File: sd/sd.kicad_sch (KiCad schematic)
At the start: 18 parts, among them J1 Micro_SD_Card_Det2, J3 STM32WORLD_BOARD, J4 STM32WORLD_CONNECTOR_1, J5 STM32WORLD_CONNECTOR_2

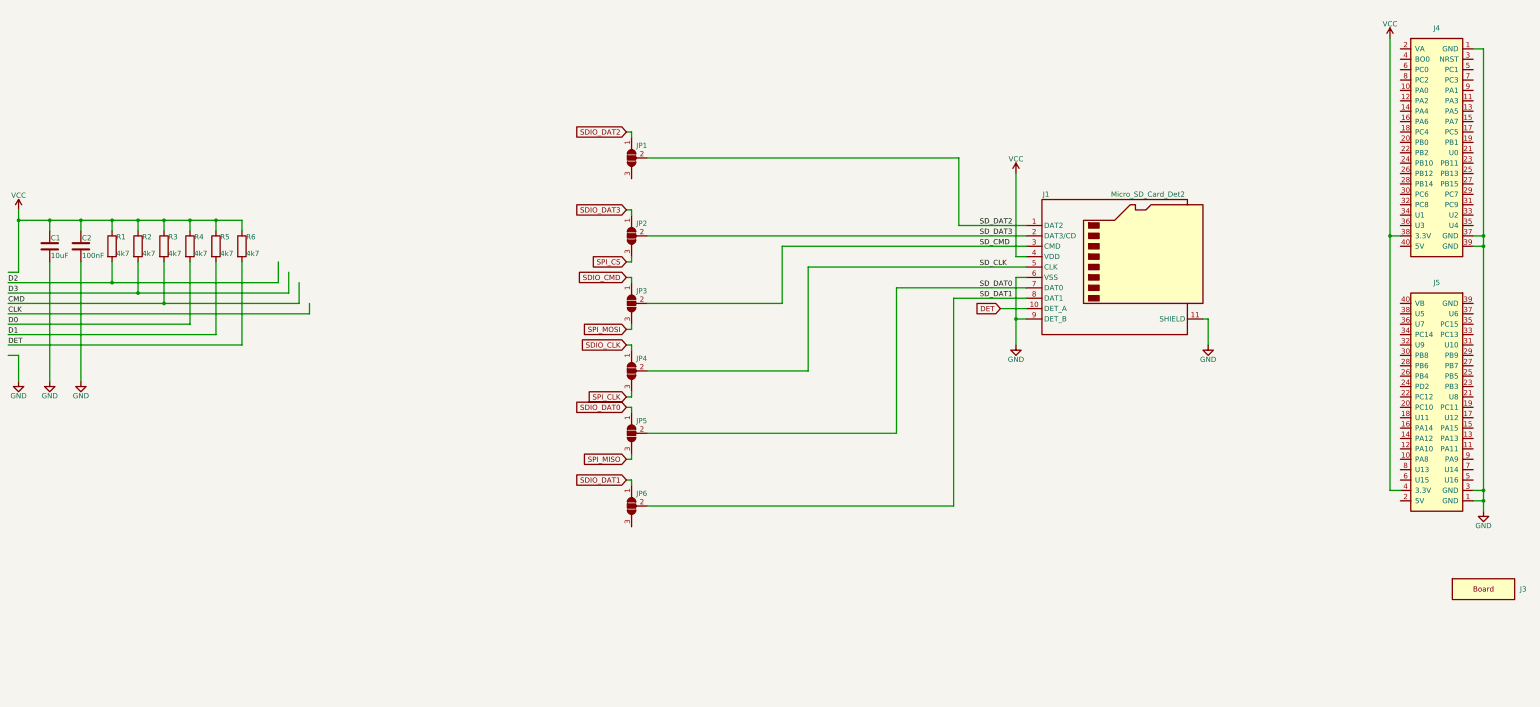
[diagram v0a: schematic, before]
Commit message: Working on sd
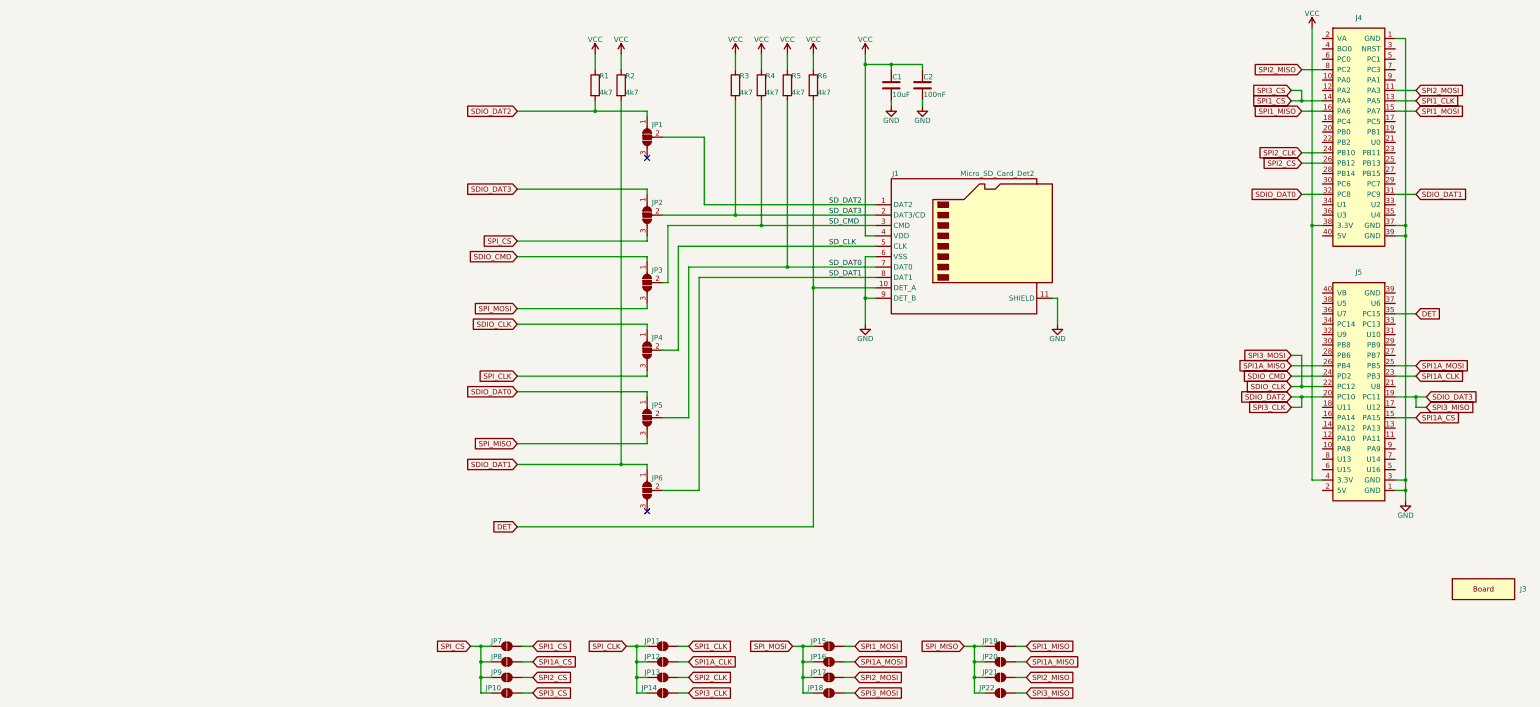
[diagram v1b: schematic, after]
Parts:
- added JP10, JP11, JP12, JP13, JP14, JP15, JP16, JP17, JP18, JP19, JP20, JP21, JP22, JP7, JP8, JP9: SolderJumper_2_Open, Jumper:SolderJumper-2_P1.3mm_Open_TrianglePad1.0x1.5mm, symbol Jumper:SolderJumper_2_Open
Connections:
- net CMD is gone; now on net SD_DAT3: R3.2
- net D0 is gone; now on net SD_CMD: R4.2
- net D1 is gone; now on net SD_DAT0: R5.2
- net D2 is gone; now on net SDIO_DAT2: R1.2
- net D3 is gone; now on net SDIO_DAT1: R2.2
- net DET: now also J5.35 (PC15)
- net SDIO_CLK: now also J5.22 (PC12), JP18.2 (B)
- net SDIO_CMD: now also J5.24 (PD2)
- net SDIO_DAT0: now also J4.32 (PC8)
- net SDIO_DAT1: now also J4.31 (PC9)
- net SDIO_DAT2: now also J5.20 (PC10), JP14.2 (B)
- net SDIO_DAT3: now also J5.19 (PC11), JP22.2 (B)
- net SPI_CLK: now also JP11.1 (A), JP12.1 (A), JP13.1 (A), JP14.1 (A)
- net SPI_CS: now also JP10.1 (A), JP7.1 (A), JP8.1 (A), JP9.1 (A)
- net SPI_MISO: now also JP19.1 (A), JP20.1 (A), JP21.1 (A), JP22.1 (A)
- net SPI_MOSI: now also JP15.1 (A), JP16.1 (A), JP17.1 (A), JP18.1 (A)
- net SPI1A_CS: now reaches J5.15 (PA15)
- net SPI1A_CS: now also JP8.2 (B)
- net SPI1A_CLK: now reaches J5.23 (PB3)
- net SPI1A_CLK: now also JP12.2 (B)
- net SPI1A_MOSI: now reaches J5.25 (PB5)
- net SPI1A_MOSI: now also JP16.2 (B)
- net SPI1A_MISO: now reaches J5.26 (PB4)
- net SPI1A_MISO: now also JP20.2 (B)
- net SPI2_MOSI: now reaches J4.11 (PA3)
- net SPI2_MOSI: now also JP17.2 (B)
- net SPI1_CLK: now reaches J4.13 (PA5)
- net SPI1_CLK: now also JP11.2 (B)
- net SPI1_CS: now reaches J4.14 (PA4)
- net SPI1_CS: now also JP10.2 (B), JP7.2 (B)
- net SPI1_MOSI: now reaches J4.15 (PA7)
- net SPI1_MOSI: now also JP15.2 (B)
- net SPI1_MISO: now reaches J4.16 (PA6)
- net SPI1_MISO: now also JP19.2 (B)
- net SPI2_CLK: now reaches J4.24 (PB10)
- net SPI2_CLK: now also JP13.2 (B)
- net SPI2_CS: now reaches J4.26 (PB12)
- net SPI2_CS: now also JP9.2 (B)
- net SPI2_MISO: now reaches J4.8 (PC2)
- net SPI2_MISO: now also JP21.2 (B)
- no-connect marks 0 -> 2
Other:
- moved on the sheet: C1, C2, J1, J4, J5, JP1, JP2, JP3, JP4, JP5, JP6, R1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
